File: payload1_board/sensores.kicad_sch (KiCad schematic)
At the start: 14 parts, among them U3 AIS328DQTR, U4 MMC5983MA, U5 I3G4250DTR

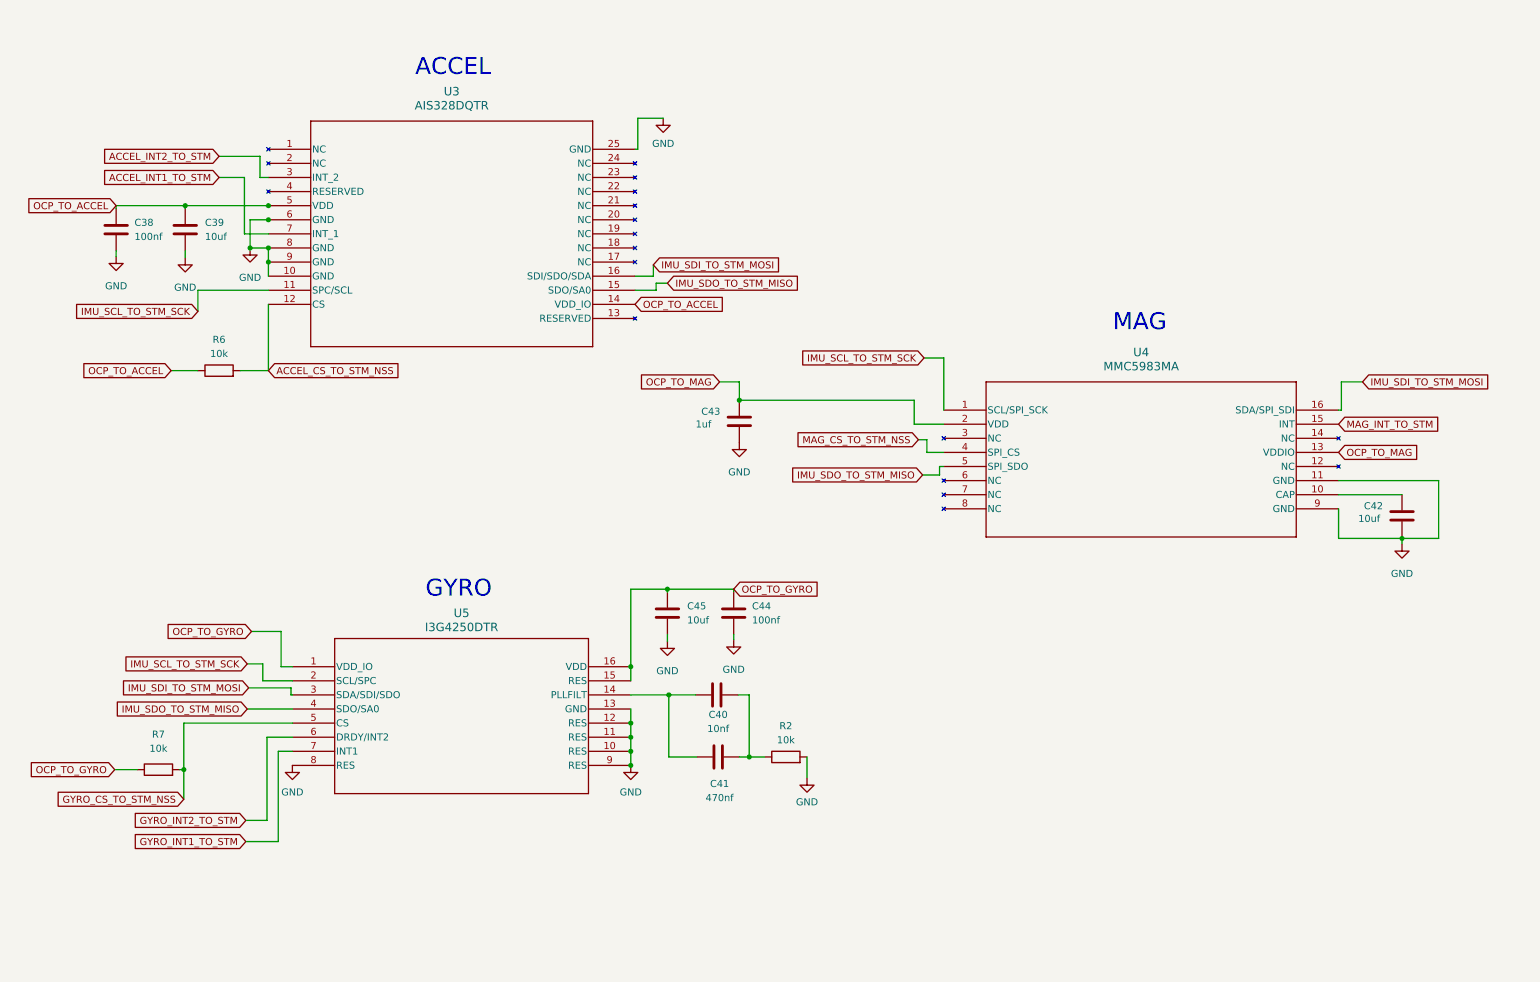
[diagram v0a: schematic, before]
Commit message: LAST UPDATE
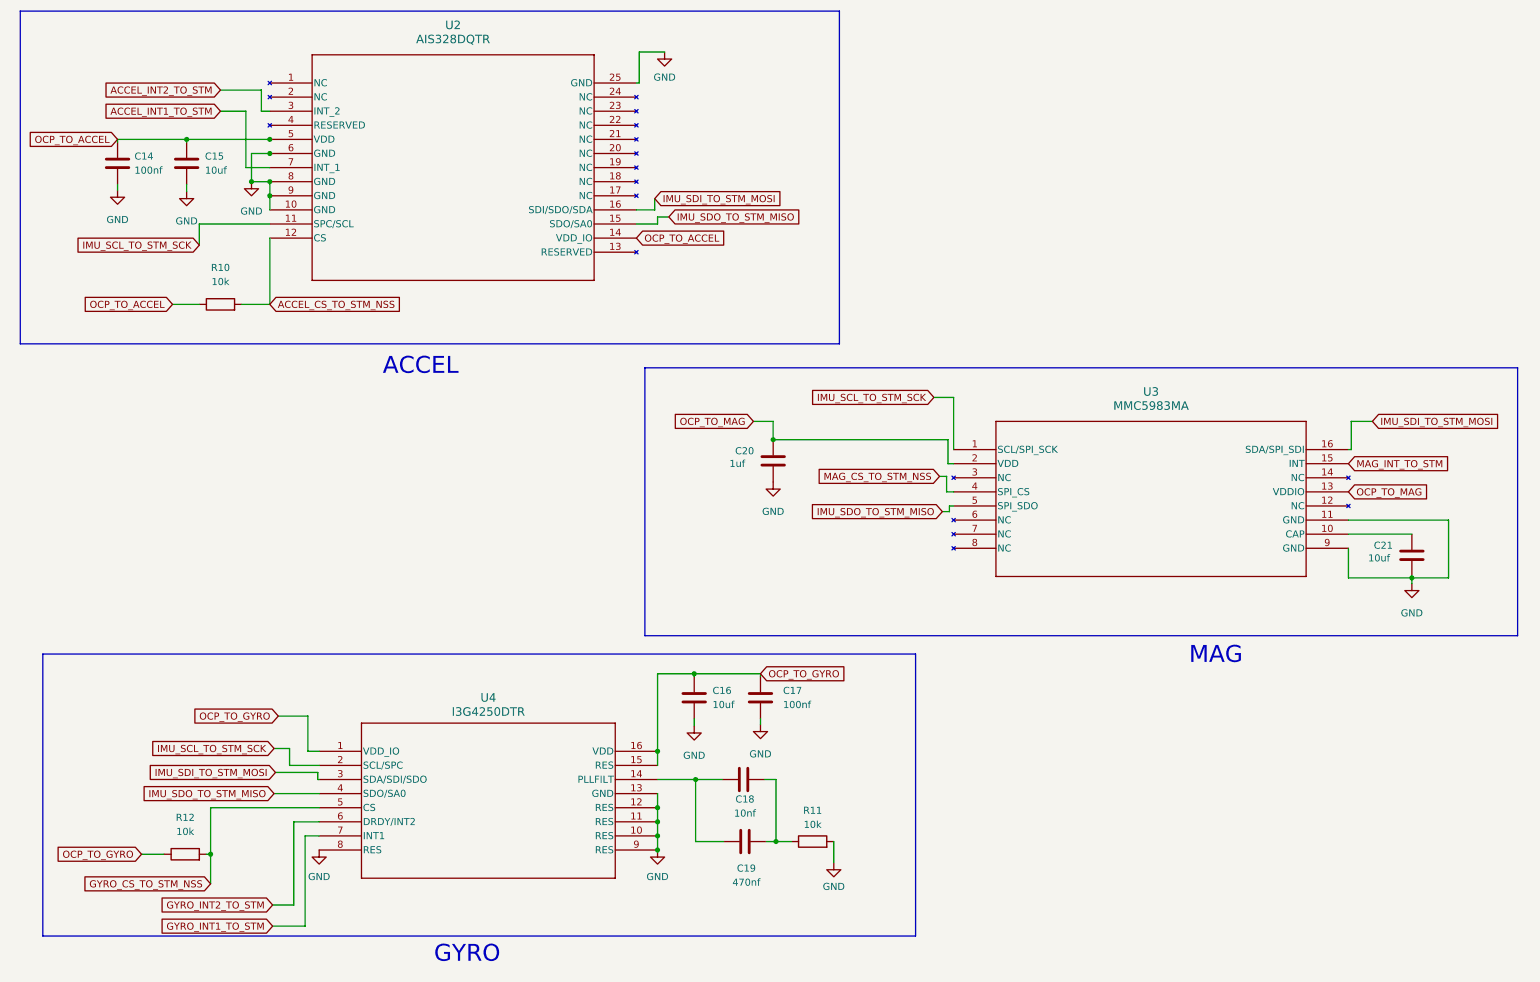
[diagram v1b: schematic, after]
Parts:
- renumbered C38 to C14, C39 to C15, C45 to C16, C44 to C17, C40 to C18, C41 to C19, C43 to C20, C42 to C21, R6 to R10, R2 to R11, R7 to R12, U3 to U2, U4 to U3, U5 to U4
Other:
- moved on the sheet: C14, C15, C16, C17, C18, C19, C20, C21, R10, R11, R12, U2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
